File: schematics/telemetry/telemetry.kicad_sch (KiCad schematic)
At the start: 12 parts, among them J1 Power, J2 PN532_Port, J4 Button_Port

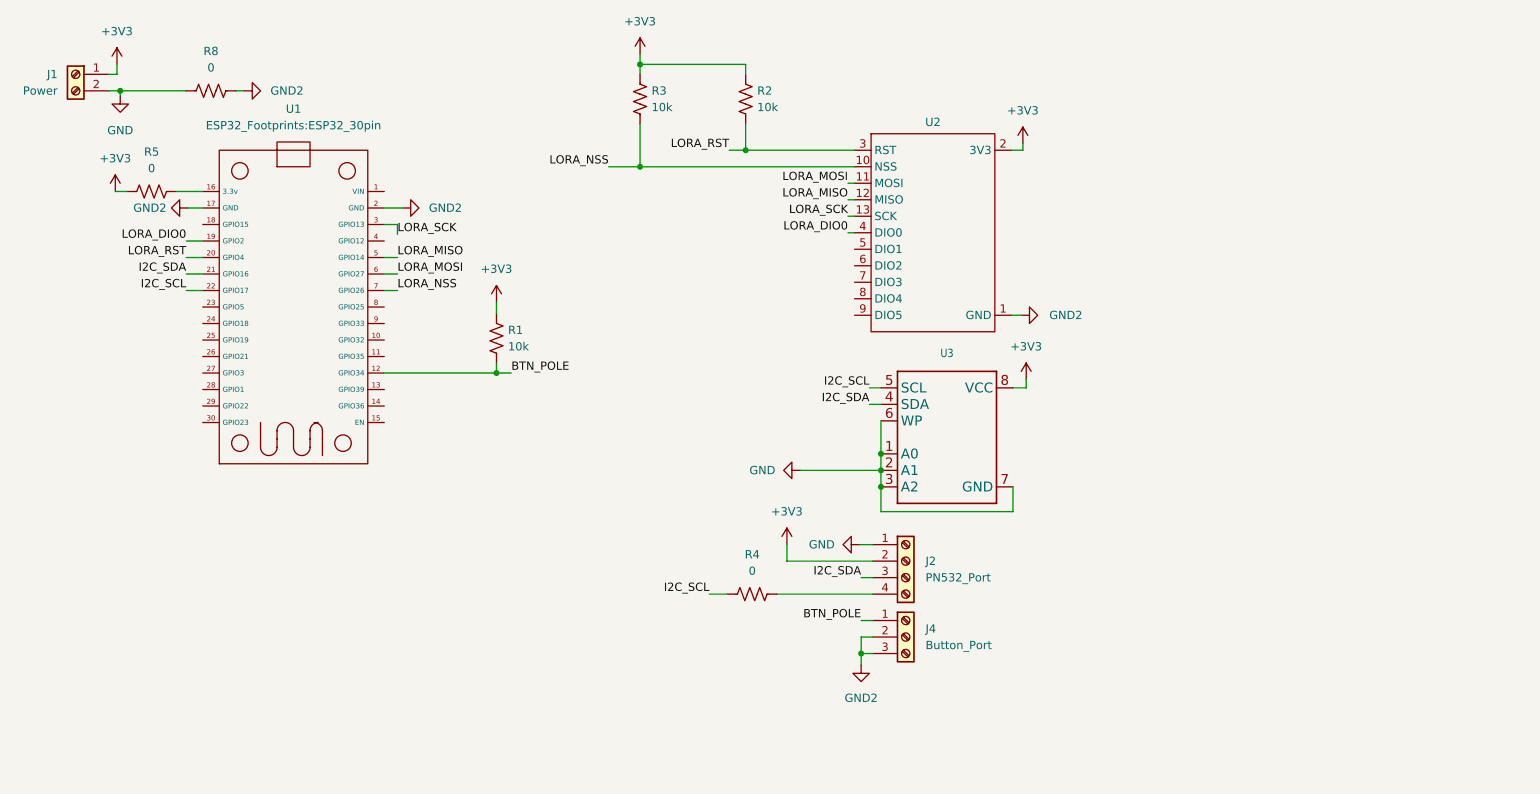
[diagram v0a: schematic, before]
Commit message: updated pcb and schematics
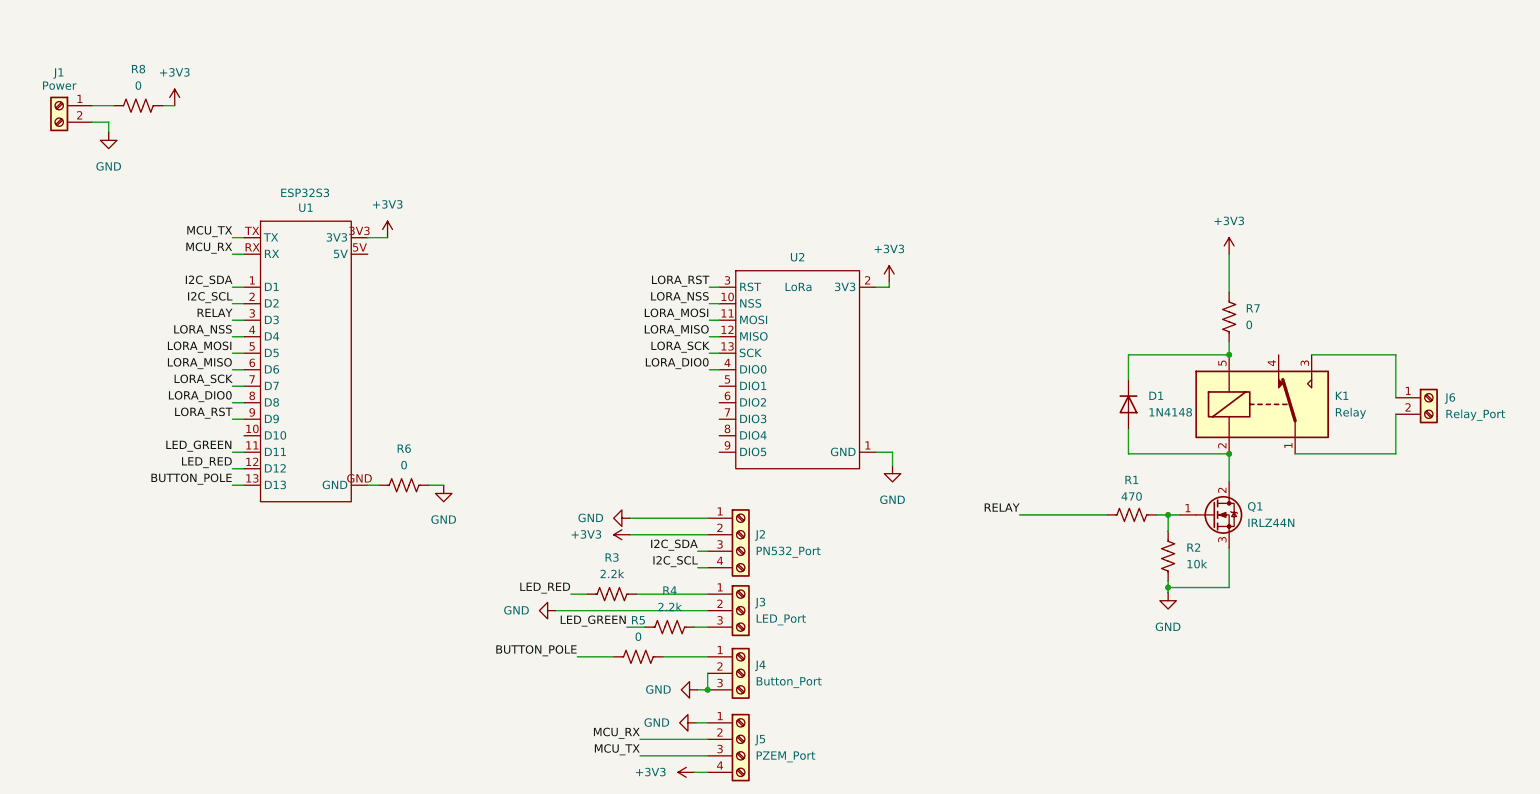
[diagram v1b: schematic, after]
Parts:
- removed U1: (no value), ESP32_Footprints:ESP32_30pin, symbol esp32_30pin_revised:ESP32_30Pin
- removed U3: (no value), LoRa_Breakout:frami2c, symbol Adafruit I2C FRAM-eagle-import:FRAM_SOIC8_I2C
- added D1: 1N4148, Diode_THT:D_DO-35_SOD27_P7.62mm_Horizontal, symbol Diode:1N4148
- added J3: LED_Port, Connector_JST:JST_EH_B3B-EH-A_1x03_P2.50mm_Vertical, symbol Connector:Screw_Terminal_01x03
- added J5: PZEM_Port, Connector_JST:JST_EH_B4B-EH-A_1x04_P2.50mm_Vertical, symbol Connector:Screw_Terminal_01x04
- added J6: Relay_Port, SH_Connectors:KF7.62_2P, symbol Connector:Screw_Terminal_01x02
- added K1: Relay, Relay_THT:Relay_SPDT_SANYOU_SRD_Series_Form_C, symbol Relay:SANYOU_SRD_Form_C
- added Q1: IRLZ44N, Package_TO_SOT_THT:TO-220-3_Vertical, symbol Transistor_FET:IRLZ44N
- added R6, R7: 0, Resistor_THT:R_Axial_DIN0207_L6.3mm_D2.5mm_P10.16mm_Horizontal, symbol Device:R_US
- added U1: ESP32S3, ESP32S3_Footprint:ESP32-S3-SuperMini, symbol esp32s3:ESP32S3_SuperMini
- J1: KiLib_Generator terminal_block/Xinya -> (none)
- J2, J4: KiLib_Generator connector/JST -> (none)
- R1: value 10k -> 470; KiLib_Generator resistor/THT -> (none)
- R2, R5: KiLib_Generator resistor/THT -> (none)
- R3: value 10k -> 2.2k; KiLib_Generator resistor/THT -> (none)
- R4: value 0 -> 2.2k; KiLib_Generator resistor/THT -> (none)
- R8: footprint Resistor_THT:R_Axial_DIN0207_L6.3mm_D2.5mm_P15.24mm_Horizontal -> Resistor_THT:R_Axial_DIN0207_L6.3mm_D2.5mm_P10.16mm_Horizontal; KiLib_Generator resistor/THT -> (none)
- U2: value (none) -> LoRa
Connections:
- net +3V3: now also R8.1, J5.4 (Pin_4), R7.1, U1.3V3; no longer J1.1 (Pin_1), R1.1, R2.1, R3.1, R5.1
- net GND: now also J4.2 (Pin_2), J4.3 (Pin_3), R2.1, U2.1 (GND), J3.2 (Pin_2), J5.1 (Pin_1), Q1.3 (S), R6.1; no longer R8.1
- net I2C_SCL: now also J2.4 (Pin_4), U1.2 (D2); no longer R4.1
- net I2C_SDA: now also U1.1 (D1)
- net LORA_DIO0: now also U1.8 (D8)
- net LORA_MISO: now also U1.6 (D6)
- net LORA_MOSI: now also U1.5 (D5)
- net LORA_NSS: now also U1.4 (D4); no longer R3.2
- net LORA_RST: now also U1.9 (D9); no longer R2.2
- net LORA_SCK: now also U1.7 (D7)
- net BUTTON_POLE: now reaches R5.2
- net BUTTON_POLE: now also U1.13 (D13)
- net LED_GREEN: now reaches R4.2
- net LED_GREEN: now also U1.11 (D11); no longer J2.4 (Pin_4)
- net BTN_POLE: no longer names the net of J4.1 (Pin_1)
- net BTN_POLE: now also R5.1; no longer R1.2
- removed net GND2: J4.2 (Pin_2), J4.3 (Pin_3), R8.2, U2.1 (GND)
- new net: R6.2, U1.GND
- new net: J3.1 (Pin_1), R3.1
- new net: J3.3 (Pin_3), R4.1
- new net: J6.1 (Pin_1), K1.3
- new net: J6.2 (Pin_2), K1.1
- new net: D1.1 (K), K1.5, R7.2
- new net: J1.1 (Pin_1), R8.2
- new net: Q1.1 (G), R1.2, R2.2
- new net: D1.2 (A), K1.2, Q1.2 (D)
- new net LED_RED: R3.2, U1.12 (D12)
- new net MCU_RX: J5.2 (Pin_2), U1.RX
- new net MCU_TX: J5.3 (Pin_3), U1.TX
- new net RELAY: R1.1, U1.3 (D3)

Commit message: adjust pad sizes for easier drilling and soldering
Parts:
- J1: footprint TerminalBlock:TerminalBlock_Xinya_XY308-2.54-2P_1x02_P2.54mm_Horizontal -> TerminalBlock:TerminalBlock_MaiXu_MX126-5.0-02P_1x02_P5.00mm
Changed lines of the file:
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@@
 			)
 		)
-		(property "Footprint" "TerminalBlock:TerminalBlock_Xinya_XY308-2.54-2P_1x02_P2.54mm_Horizontal"
+		(property "Footprint" "TerminalBlock:TerminalBlock_MaiXu_MX126-5.0-02P_1x02_P5.00mm"
 			(at 21.59 29.972 0)
 			(hide yes)
